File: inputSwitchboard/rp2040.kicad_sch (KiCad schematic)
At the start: 6 parts, among them U2 RP2040, U9 TXS0108EPW

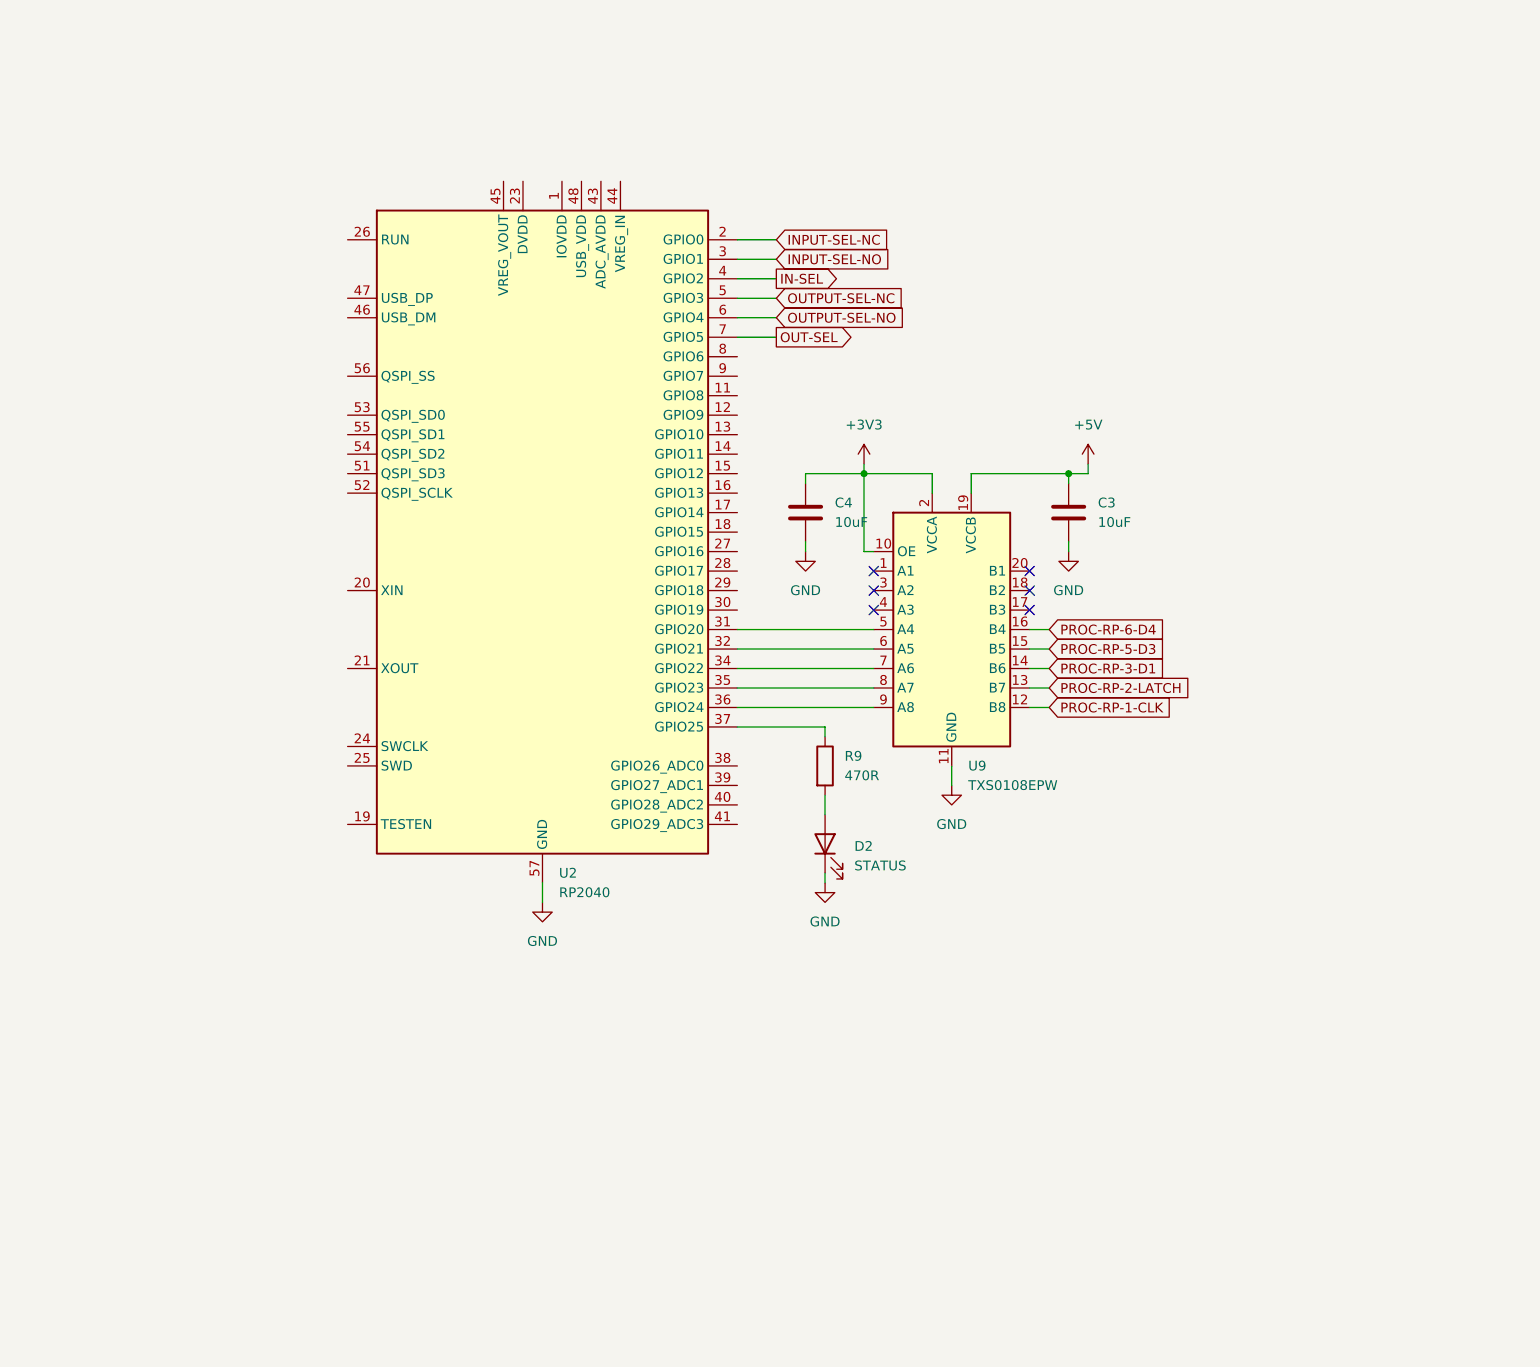
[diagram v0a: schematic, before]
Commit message: finished schematic
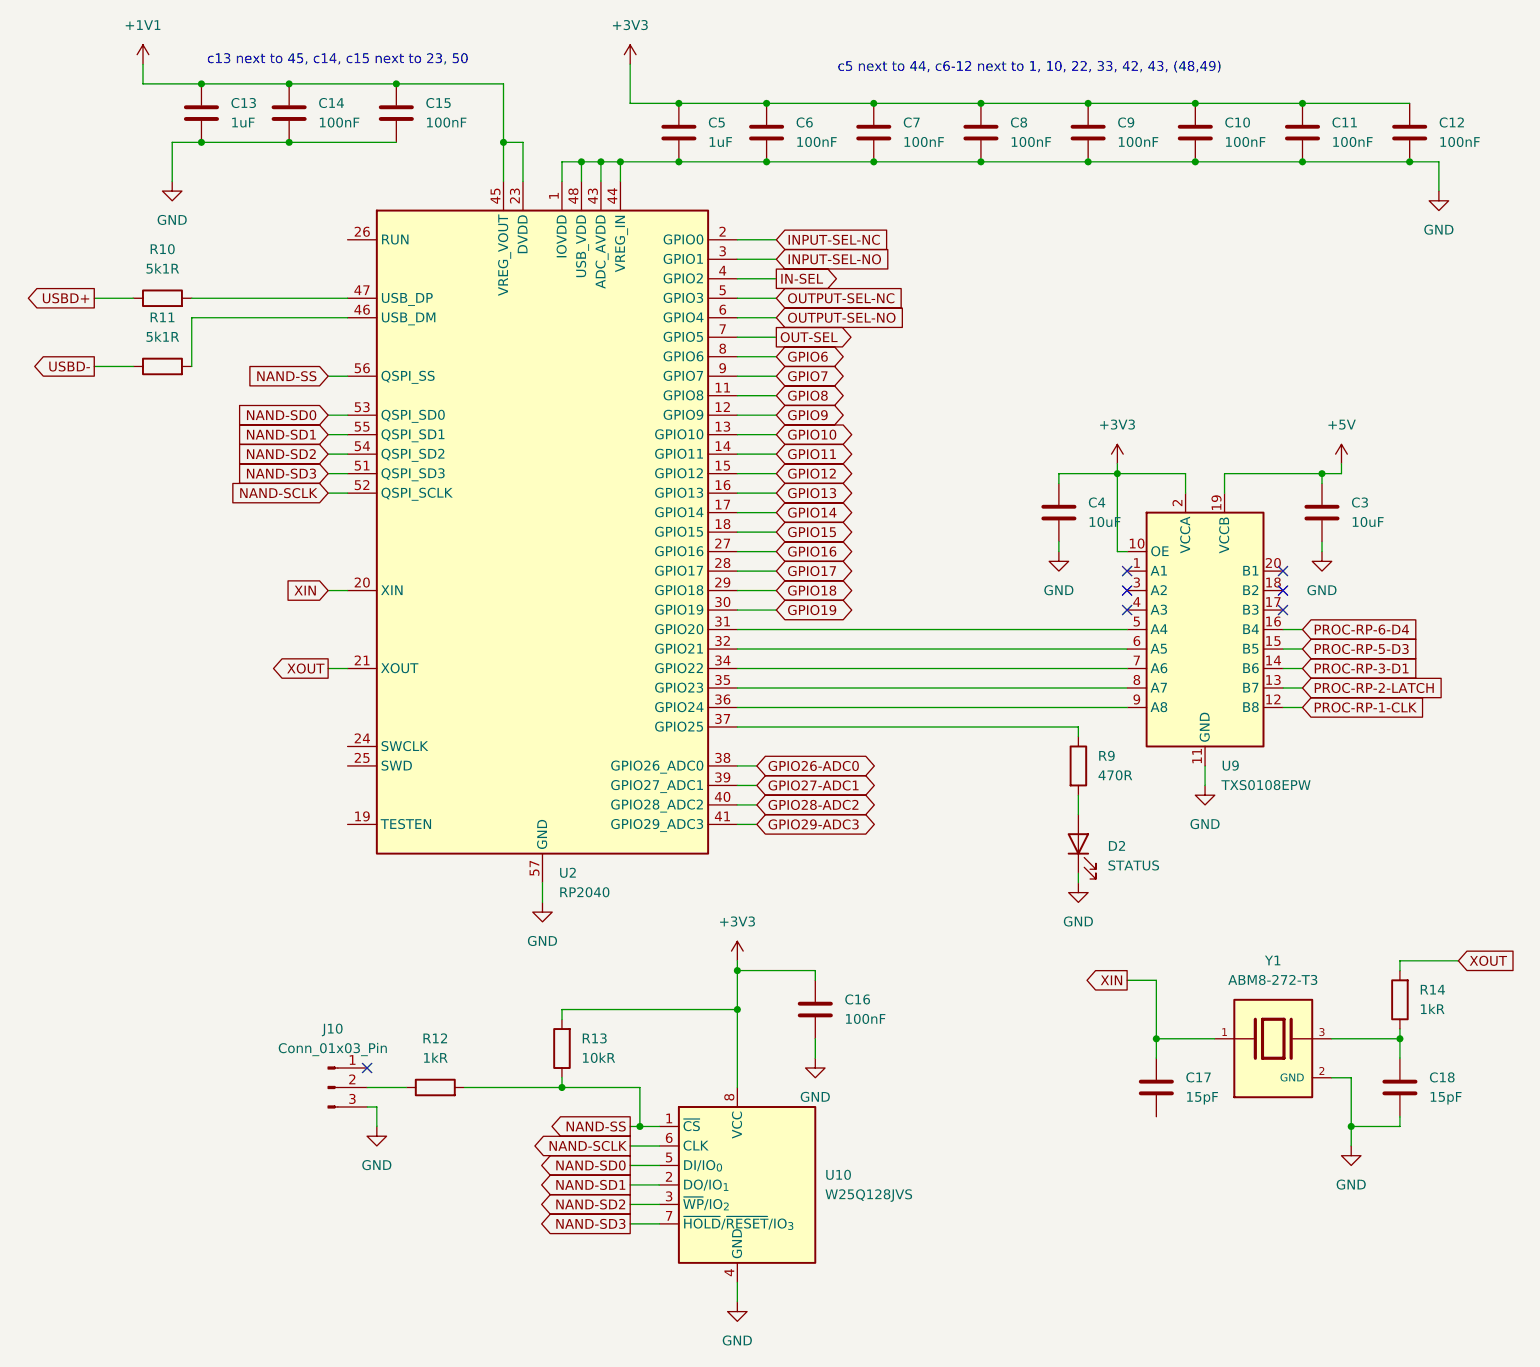
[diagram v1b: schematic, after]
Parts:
- added C10, C11, C12, C14, C15, C16, C6, C7, C8, C9: 100nF, Capacitor_SMD:C_0201_0603Metric, symbol Device:C
- added C13, C5: 1uF, Capacitor_SMD:C_0201_0603Metric, symbol Device:C
- added C17, C18: 15pF, Capacitor_SMD:C_0201_0603Metric, symbol Device:C
- added J10: Conn_01x03_Pin, Connector:FanPinHeader_1x03_P2.54mm_Vertical, symbol Connector:Conn_01x03_Pin
- added R10, R11: 5k1R, Resistor_SMD:R_0603_1608Metric, symbol Device:R
- added R12, R14: 1kR, Resistor_SMD:R_0603_1608Metric, symbol Device:R
- added R13: 10kR, Resistor_SMD:R_0603_1608Metric, symbol Device:R
- added U10: W25Q128JVS, Package_SO:SOIC-8_5.3x5.3mm_P1.27mm, symbol Memory_Flash:W25Q128JVS
- added Y1: ABM8-272-T3, ABM8-272-T3:XTAL_ABM8-272-T3, symbol ABM8-272-T3:ABM8-272-T3
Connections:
- net +3V3: now also C10.1, C11.1, C12.1, C16.1, C5.1, C6.1, C7.1, C8.1, C9.1, R13.2, U10.8 (VCC)
- net GND: now also U2.1 (IOVDD), U2.10 (IOVDD), U2.22 (IOVDD), U2.33 (IOVDD), U2.42 (IOVDD), U2.43 (ADC_AVDD), U2.44 (VREG_IN), U2.48 (USB_VDD), U2.49 (IOVDD), C10.2, C11.2, C12.2, C13.2, C14.2, C15.2, C16.2, C18.2, C5.2, C6.2, C7.2, C8.2, C9.2, J10.3 (Pin_3), U10.4 (GND), Y1.2 (GND), Y1.4 (GND)
- net GPIO8: now reaches U2.11 (GPIO8)
- net GPIO9: now reaches U2.12 (GPIO9)
- net GPIO10: now reaches U2.13 (GPIO10)
- net GPIO11: now reaches U2.14 (GPIO11)
- net GPIO12: now reaches U2.15 (GPIO12)
- net GPIO13: now reaches U2.16 (GPIO13)
- net GPIO14: now reaches U2.17 (GPIO14)
- net GPIO15: now reaches U2.18 (GPIO15)
- net XIN: now reaches U2.20 (XIN)
- net XIN: now also C17.1, Y1.1
- net XOUT: now reaches U2.21 (XOUT)
- net XOUT: now also R14.2
- net +1V1: now reaches U2.23 (DVDD), U2.50 (DVDD)
- net +1V1: now also U2.45 (VREG_VOUT), C13.1, C14.1, C15.1
- net GPIO16: now reaches U2.27 (GPIO16)
- net GPIO17: now reaches U2.28 (GPIO17)
- net GPIO18: now reaches U2.29 (GPIO18)
- net GPIO19: now reaches U2.30 (GPIO19)
- net GPIO26-ADC0: now reaches U2.38 (GPIO26_ADC0)
- net GPIO27-ADC1: now reaches U2.39 (GPIO27_ADC1)
- net GPIO28-ADC2: now reaches U2.40 (GPIO28_ADC2)
- net GPIO29-ADC3: now reaches U2.41 (GPIO29_ADC3)
- net at U2.46 (USB_DM): now also R11.2
- net at U2.47 (USB_DP): now also R10.2
- net NAND-SD3: now reaches U2.51 (QSPI_SD3)
- net NAND-SD3: now also U10.7 (~{HOLD}/~{RESET}/IO_{3})
- net NAND-SCLK: now reaches U2.52 (QSPI_SCLK)
- net NAND-SCLK: now also U10.6 (CLK)
- net NAND-SD0: now reaches U2.53 (QSPI_SD0)
- net NAND-SD0: now also U10.5 (DI/IO_{0})
- net NAND-SD2: now reaches U2.54 (QSPI_SD2)
- net NAND-SD2: now also U10.3 (~{WP}/IO_{2})
- net NAND-SD1: now reaches U2.55 (QSPI_SD1)
- net NAND-SD1: now also U10.2 (DO/IO_{1})
- net NAND-SS: now reaches U2.56 (QSPI_SS)
- net NAND-SS: now also R12.2, R13.1, U10.1 (~{CS})
- net GPIO6: now reaches U2.8 (GPIO6)
- net GPIO7: now reaches U2.9 (GPIO7)
- new net: J10.2 (Pin_2), R12.1
- new net: C18.1, R14.1, Y1.3
- new net USBD+: R10.1
- new net USBD-: R11.1
- no-connect marks 6 -> 7
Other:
- note added: "c13 next to 45, c14, c15 next to 23, 50"
- note added: "c5 next to 44, c6-12 next to 1, 10, 22, 33, 42, 43, (48,49)"
- moved on the sheet: C3, C4, D2, R9, U9
